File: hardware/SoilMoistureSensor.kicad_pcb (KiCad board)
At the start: 2 copper layers, 43 x 89.5 mm, 36 parts, among them J1 Conn_01x02, J2 Conn_01x04, J3 Conn_01x02, Q1 AO3401A, SW1 SW_Push, SW2 SW_Push, U1 BQ25570, U2 ESP32-C3-WROOM-02, U3 TLC555xD

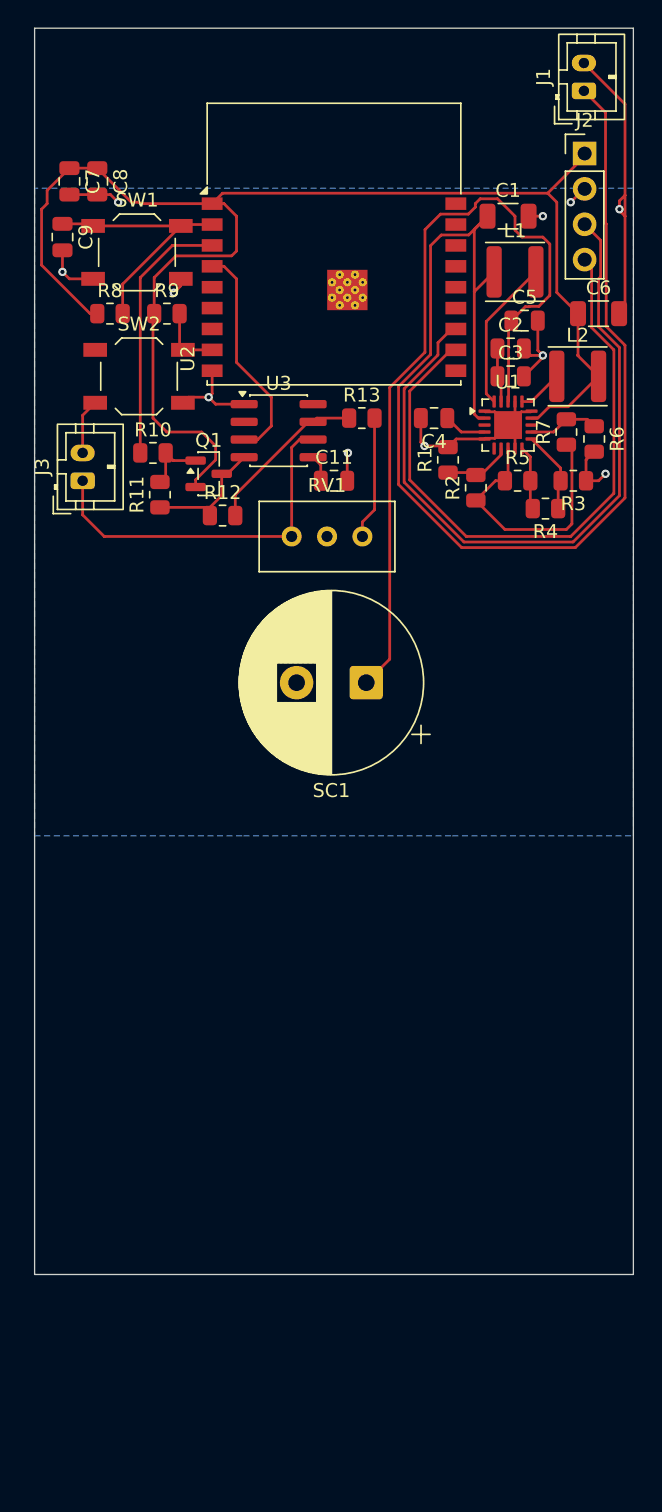
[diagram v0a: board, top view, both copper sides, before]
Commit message: astra redesigned then ran out of usage
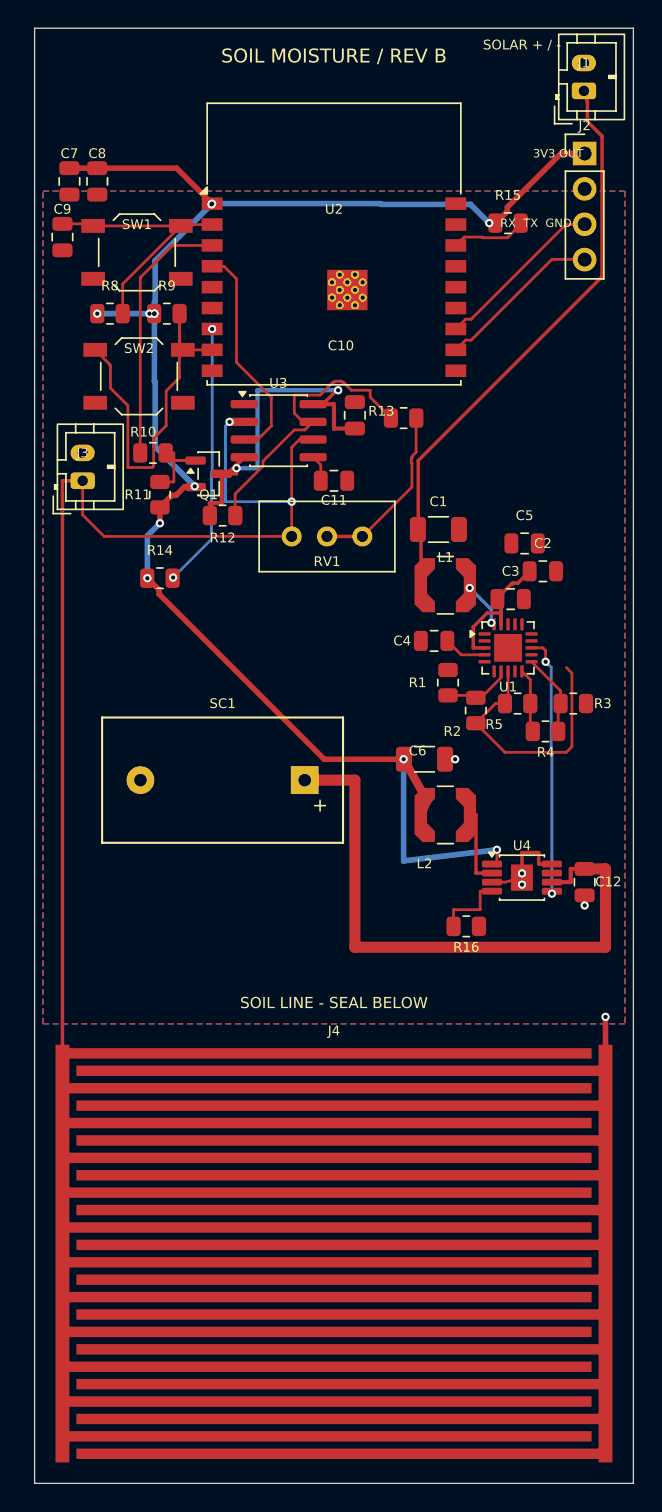
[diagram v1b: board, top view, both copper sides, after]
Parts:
- removed R6: 4.75M 1%, Resistor_SMD:R_0805_2012Metric
- removed R7: 8.25M 1%, Resistor_SMD:R_0805_2012Metric
- added C10: 100nF 10V, Capacitor_SMD:C_0805_2012Metric, F.Cu at (118.0, 74.8)
- added C12: 10uF 10V X7R, Capacitor_SMD:C_0805_2012Metric, F.Cu at (134.5, 108.3)
- added J4: PCB capacitive probe, SoilProbe:SoilProbe_IDC_40x30mm, F.Cu at (116.5, 135.0)
- added R14: 10k, Resistor_SMD:R_0805_2012Metric, F.Cu at (104.0, 86.5)
- added R15: 10k, Resistor_SMD:R_0805_2012Metric, F.Cu at (129.0, 61.0)
- added R16: 52.3k 1%, Resistor_SMD:R_0805_2012Metric, F.Cu at (126.0, 111.5)
- added U4: TPS62842DGRR, Package_SO:HVSSOP-8-1EP_3x3mm_P0.65mm_EP1.57x1.89mm, F.Cu at (130.0, 108.0)
- C1, C2: value 4.7uF -> 4.7uF 10V X7R
- C11: value 100nF -> 10nF
- C3: value 0.1uF -> 100nF 10V
- C4: value 10nF -> 10nF C0G 5%
- C5, C8, C9: value 100nF -> 100nF 10V
- C6: value 22uF -> 10uF 10V X7R
- C7: value 10uF -> 10uF 10V X7R
- L1: value 22uH -> 22uH / Isat >= 0.4A; footprint Inductor_SMD:L_APV_ANR4030 -> Inductor_SMD:L_Coilcraft_LPS4018
- L2: value 10uH -> 2.2uH / Isat >= 1.5A; footprint Inductor_SMD:L_APV_ANR4030 -> Inductor_SMD:L_Coilcraft_LPS4018
- R1: value 3.01M 1% -> 4.75M 1%
- R12: value 1k -> 10k
- R13: value 4.7k -> 47k
- R2: value 10.0M 1% -> 8.25M 1%
- RV1: value 10k trim -> 100k trim
- SC1: value 3F 5.5V Supercap -> 3F 5.4V PHV-5R4V305-R; footprint Capacitor_THT:CP_Radial_D13.0mm_P5.00mm -> SoilProbe:CP_Eaton_PHV_3F_Vertical_P11.8mm
- moved C6 34.4 mm to (123.0, 99.5)
- moved L2 32.9 mm to (124.5, 103.5), turned to 180 degrees
- moved C1 23.0 mm to (124.0, 83.0)
- moved L1 23.0 mm to (124.5, 87.0)
- moved C2 16.2 mm to (131.5, 86.0)
- moved C3 16.0 mm to (129.2, 88.0)
- moved C4 16.0 mm to (123.7, 91.0)
- moved C5 16.0 mm to (130.2, 84.0)
- moved R1 16.0 mm to (124.7, 94.0)
- moved R2 16.0 mm to (126.7, 96.0)
- moved R3 16.0 mm to (133.7, 95.5)
- moved R4 16.0 mm to (131.7, 97.5)
- moved R5 16.0 mm to (129.7, 95.5)
- moved U1 16.0 mm to (129.0, 91.5)
- moved SC1 12.5 mm to (108.5, 101.0), turned to 0 degrees
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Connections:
- C1 pad 2: GND -> /GND
- C11 pad 2: GND -> /GND
- C2 pad 2: GND -> /GND
- C3 pad 2: GND -> /GND
- C4 pad 2: GND -> /GND
- C5 pad 2: GND -> /GND
- C6 pad 1: +3V3 -> /+3V3
- C6 pad 2: GND -> /GND
- C7 pad 1: +3V3 -> /+3V3
- C7 pad 2: GND -> /GND
- C8 pad 1: +3V3 -> /+3V3
- C8 pad 2: GND -> /GND
- C9 pad 2: GND -> /GND
- J1 pad 2: GND -> /GND
- J2 pad 1: +3V3 -> /+3V3
- J2 pad 2: GND -> /GND
- J3 pad 2: GND -> /GND
- L2 pad 1: /LBUCK -> /BUCK_SW
- L2 pad 2: +3V3 -> /+3V3
- Q1 pad 2: +3V3 -> /+3V3
- R1 pad 2: GND -> /GND
- R11 pad 1: /VCC_SENSOR -> /+3V3
- R3 pad 1: GND -> /GND
- R8 pad 1: +3V3 -> /+3V3
- R9 pad 1: +3V3 -> /+3V3
- SC1 pad 2: GND -> /GND
- SW1 pad 2: GND -> /GND
- SW2 pad 2: GND -> /GND
- U1 pad 1: GND -> /GND
- U1 pad 12: /VOUT_SET_N -> /GND
- U1 pad 14: +3V3 -> unconnected-(U1-VOUT-Pad14)
- U1 pad 15: GND -> /GND
- U1 pad 16: /LBUCK -> unconnected-(U1-LBUCK-Pad16)
- U1 pad 17: GND -> /GND
- U1 pad 21: GND -> /GND
- U1 pad 5: GND -> /GND
- U1 pad 6: /BAT_OK -> /GND
- U1 pad 9: GND -> /GND
- U2 pad 1: +3V3 -> /+3V3
- U2 pad 16: unconnected-(U2-IO2-Pad16) -> /GPIO2_BOOT
- U2 pad 19: GND -> /GND
- U2 pad 7: unconnected-(U2-IO8-Pad7) -> /GPIO8_BOOT
- U2 pad 9: GND -> /GND
- U3 pad 1: GND -> /GND
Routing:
- net /+3V3: track 0.00 -> 121.0 mm, vias 0 -> 12
- net +3V3: track 104.0 -> 0.00 mm
- net GND: track 73.1 -> 0.00 mm, vias 11 -> 0
- net /OSC_RC: track 26.3 -> 79.9 mm, vias 0 -> 2
- net /VIN_DC: track 90.6 -> 41.7 mm
- net /ESP_TXD: track 52.0 -> 12.4 mm
- net /ESP_RXD: track 46.2 -> 12.0 mm
- net /GPIO9_BOOT: track 4.80 -> 27.8 mm
- net /GPIO8_BOOT: track 0.00 -> 19.1 mm, vias 0 -> 2
- net /BAT_OK: track 0.00 -> 19.0 mm, vias 0 -> 2
- net /VCC_SENSOR: track 8.46 -> 27.3 mm, vias 0 -> 2
- net /VBAT: track 59.4 -> 44.0 mm
- net /GND: track 0.00 -> 10.4 mm, vias 0 -> 5
- net /OSC_RC_DISCH: track 11.9 -> 21.2 mm
- net /LBOOST: track 11.0 -> 3.61 mm, vias 0 -> 2
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- added copper zone on B.Cu, net /GND
- added copper zone on F.Cu, net /GND
- removed copper zone on B.Cu, net GND
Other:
- board size 43 x 89.5 mm -> 43 x 104.5 mm
- board text added: "3V3 OUT"
- board text added: "RX TX GND"
- board text added: "SOIL LINE - SEAL BELOW"
- board text added: "SOIL MOISTURE / REV B"
- board text added: "SOLAR + / -"
